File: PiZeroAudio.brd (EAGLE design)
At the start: 65.1 x 30.2 mm, 53 parts, among them CN1 1X4-BIG, CON1 RPI-ZERO, J1 1X2-3.5MM, U1 TXB0104PWR, U2 LSM6DS33, U3 NC7WZ16, U4 TPA3144D2PWPR

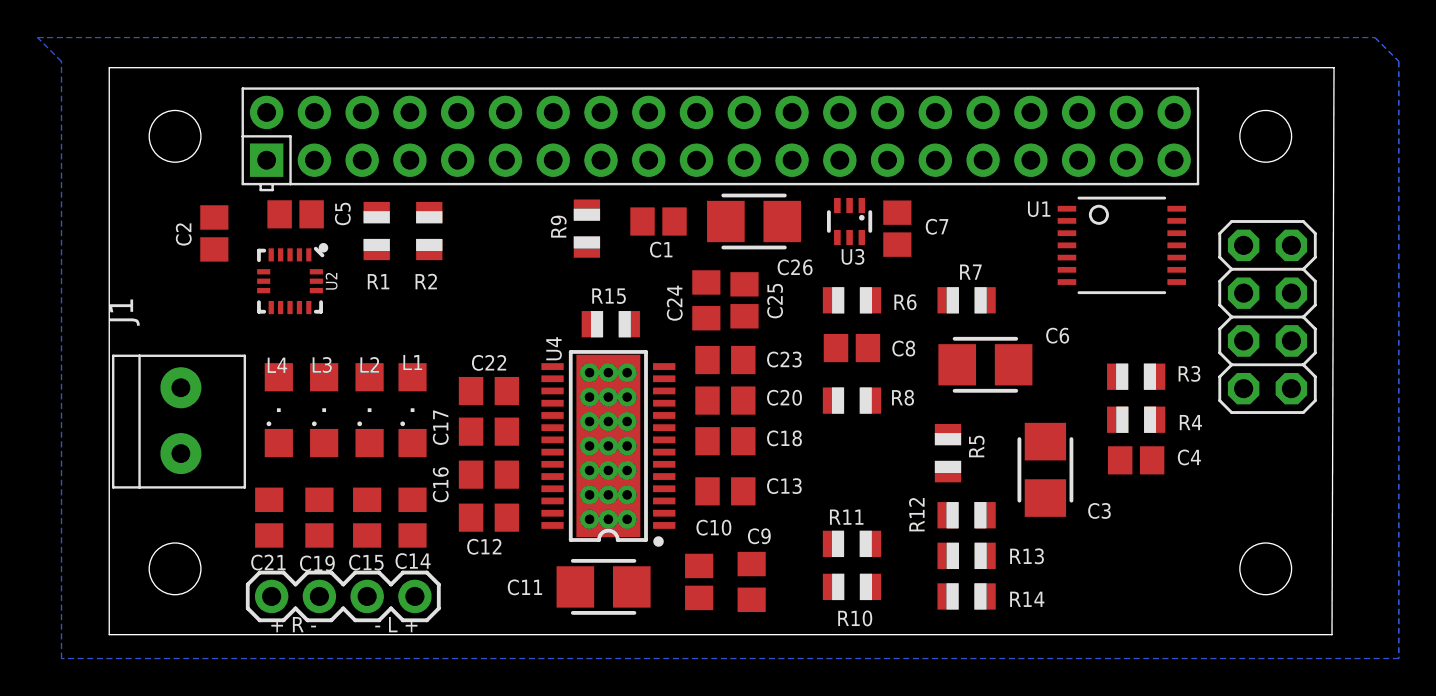
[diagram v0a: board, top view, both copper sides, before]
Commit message: Applied star Power
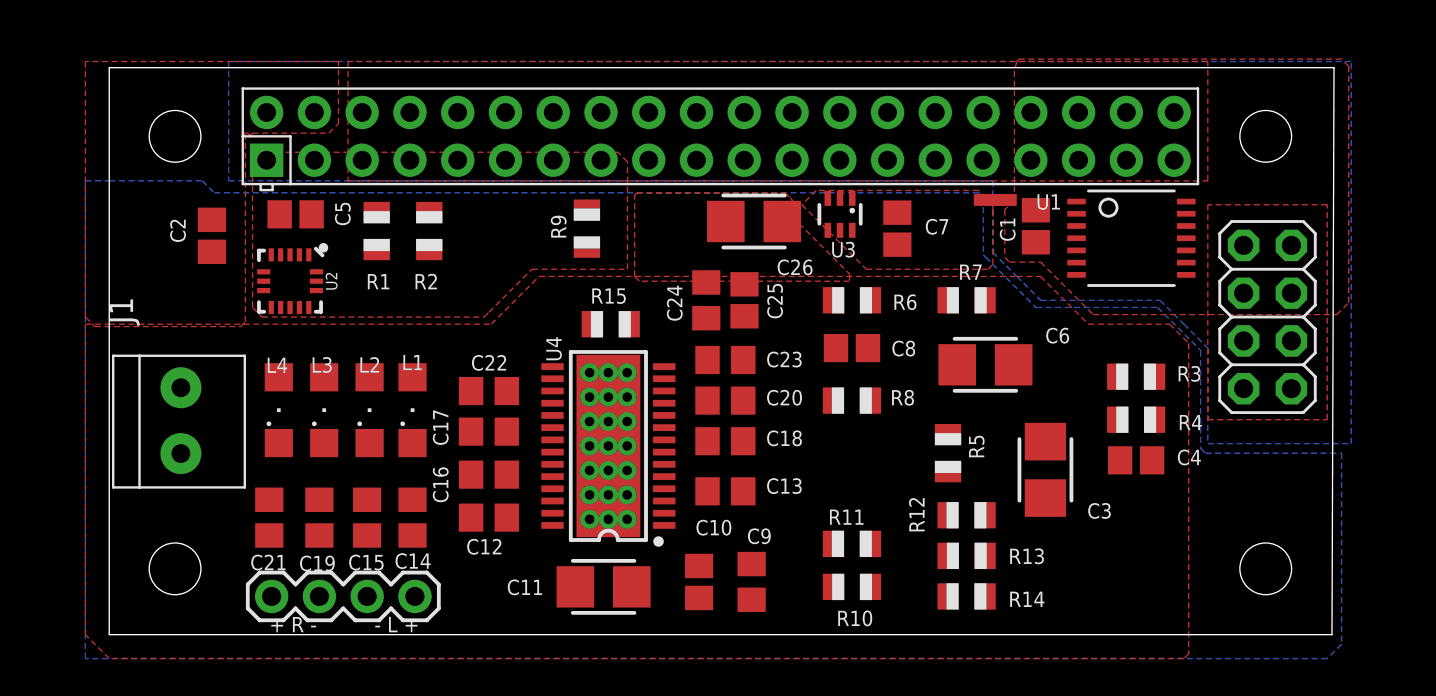
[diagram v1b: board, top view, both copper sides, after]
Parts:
- added SH1, SH2: SHORT, HappyBrackets:SHORT
- moved C1 20.1 mm to (-29.5, 23.0), turned to 270 degrees
- moved U3 0.64 mm to (-39.9, 23.6)
- moved U1 0.63 mm to (-24.4, 22.4)
- moved C2 0.18 mm to (-73.3, 22.5), turned to 90 degrees
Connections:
- new net AGND: C10.2, C11.-, C13.2, C14.2, C15.1, C18.2, C19.2, C20.2, C21.1, C23.2, C24.2, C25.2, C26.-, C4.2, C7.2, C8.2, C9.2, J1.1, R10.2, R12.2, R4.1, R5.1, R7.1, R8.1, SH2.AN, U4.10, U4.13, U4.19, U4.24
- new net AN3V3: C7.1, SH1.AN, U3.5
- net +3V3: now also SH1.DIG; no longer C7.1, U3.5
- net GND: now also SH2.DIG; no longer C10.2, C11.-, C13.2, C14.2, C15.1, C18.2, C19.2, C20.2, C21.1, C23.2, C24.2, C25.2, C26.-, C4.2, C7.2, C8.2, C9.2, J1.1, R10.2, R12.2, R4.1, R5.1, R7.1, R8.1, U4.10, U4.13, U4.19, U4.24
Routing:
- added copper zone on layer 1, net +3V3
- added copper zone on layer 1, net +5V
- added copper zone on layer 1, net AN3V3
- added copper zone on layer 16, net ANGND
